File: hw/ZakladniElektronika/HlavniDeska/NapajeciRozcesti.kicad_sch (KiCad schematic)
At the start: 32 parts, among them Q1 Q_PMOS_DGS, Q2 Q_PMOS_DGS, U11 150k, U12 100k, U13 TPS61088RHLR, U14 100k, U15 2N7002, U16 LD39200, U17 33n, U18 150k, U19 22u, U20 4.7u, U21 10uf, U22 22u, U23 100k, U24 2N7002, U25 3.92k, U26 10n, U27 2.2u, U28 22u, U29 100p, U3 22u, U30 56k, U31 17.4k, U32 150k, U5 10uf, U6 100n, U7 1.2u, U8 4.7u, U9 100n

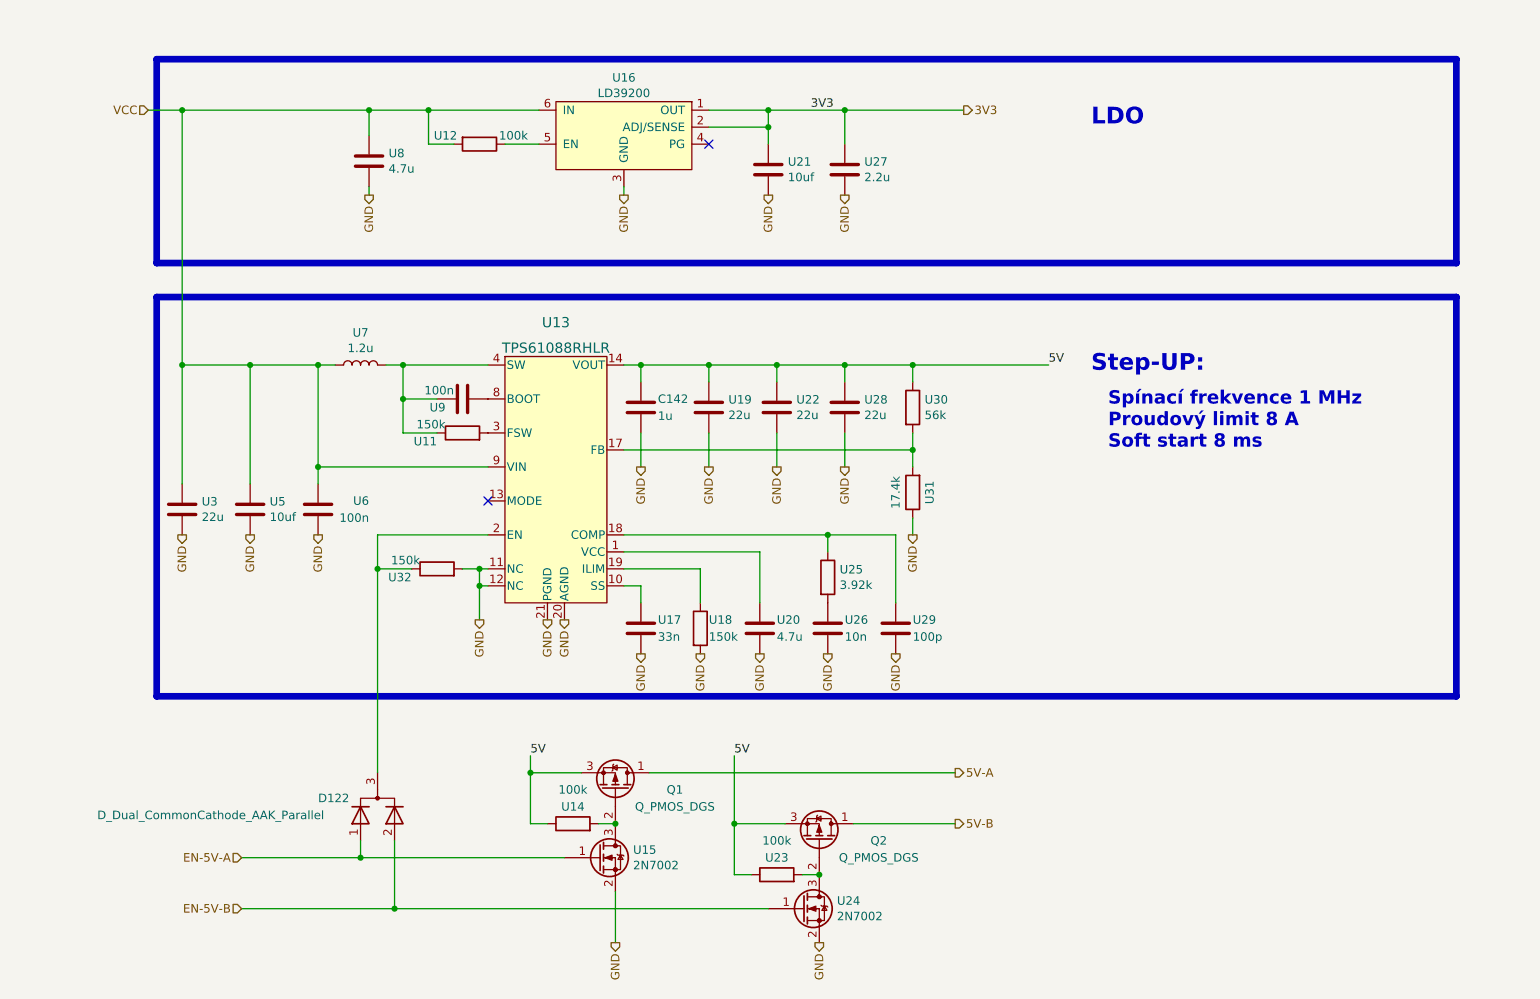
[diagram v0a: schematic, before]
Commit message: WIP
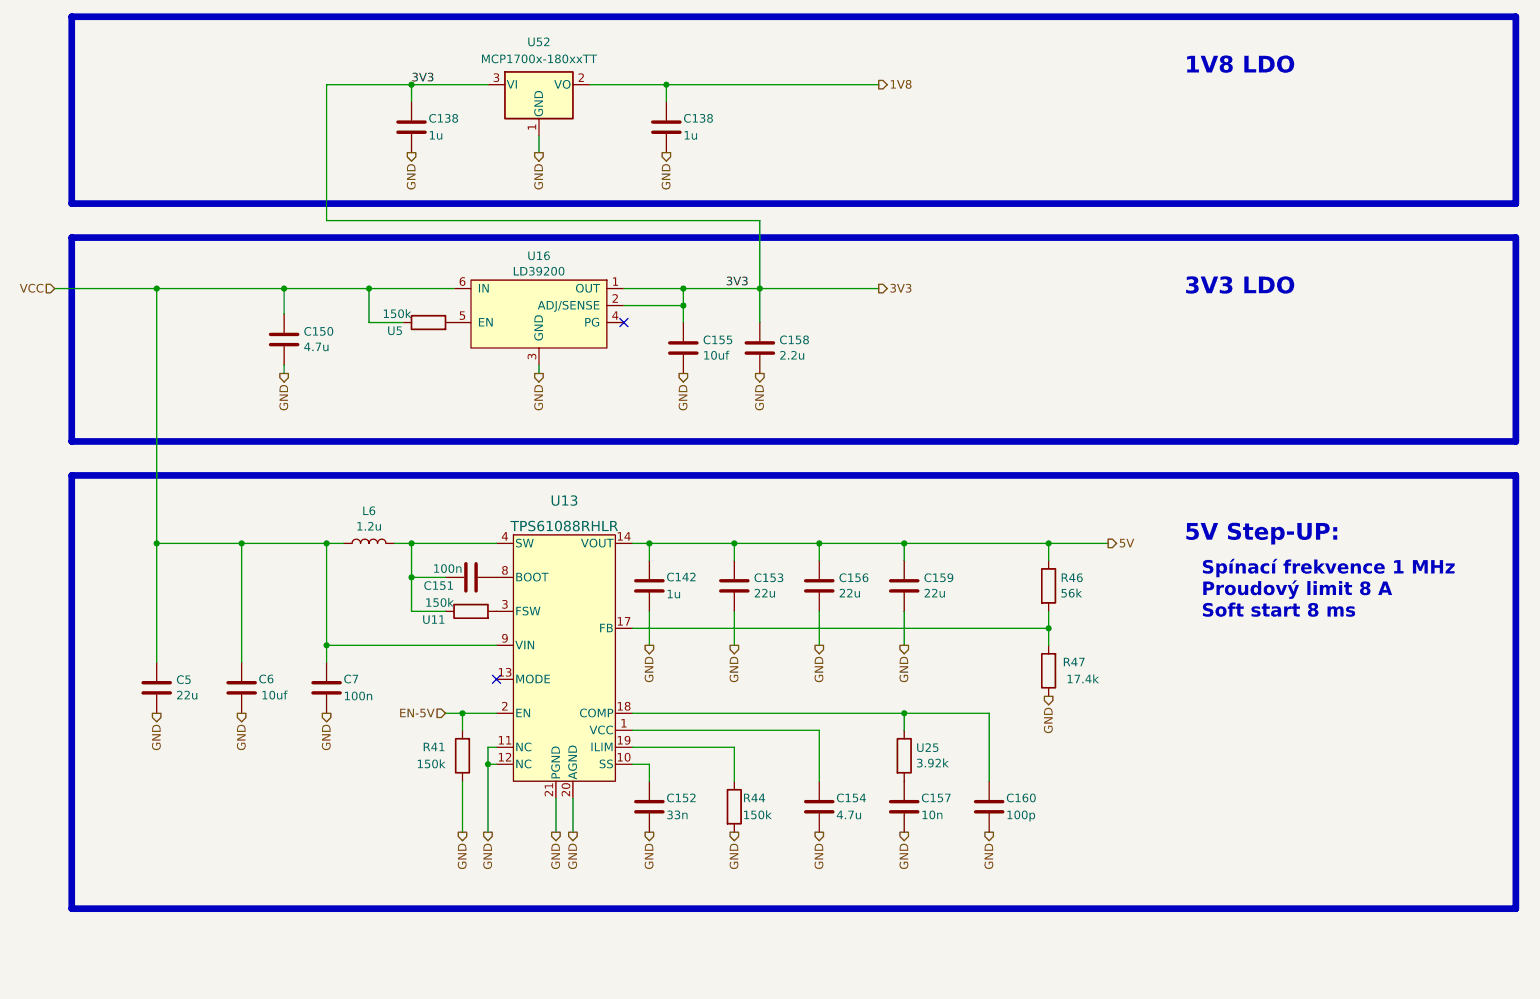
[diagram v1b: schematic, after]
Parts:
- removed D122: D_Dual_CommonCathode_AAK_Parallel, Package_TO_SOT_SMD:SOT-723, symbol Device:D_Dual_CommonCathode_AAK_Parallel
- removed Q1, Q2: Q_PMOS_DGS, RBCX:JMSL0302AU, symbol Device:Q_PMOS_DGS
- removed U12, U14, U23: 100k, Resistor_SMD:R_0402_1005Metric, symbol B.B-rescue:R-Device-B.B-rescue-B.B-rescue
- removed U15, U24: 2N7002, Package_TO_SOT_SMD:SOT-23, symbol B.B-rescue:2N7002-Transistor_FET-B.B-rescue-B.B-rescue
- added C138 (x2): 1u, Resistor_SMD:R_0402_1005Metric, symbol Device:C
- added U5: 150k, Resistor_SMD:R_0402_1005Metric, symbol B.B-rescue:R-Device-B.B-rescue-B.B-rescue
- added U52: MCP1700x-180xxTT, Package_TO_SOT_SMD:SOT-23, symbol Regulator_Linear:MCP1700x-180xxTT
- C142: Basic/Extended (none) -> E; LCSC C52923 -> C1518208; info (none) -> 50V, X7R
- C150: renamed from U8; symbol B.B-rescue:C-Device-B.B-rescue-B.B-rescue -> Device:C
- C151: renamed from U9; symbol B.B-rescue:C-Device-B.B-rescue-B.B-rescue -> Device:C; Basic/Extended (none) -> B; LCSC C1525 -> C307331; info (none) -> 50V, X7R
- C152: renamed from U17; symbol B.B-rescue:C-Device-B.B-rescue-B.B-rescue -> Device:C
- C153: renamed from U19; symbol B.B-rescue:C-Device-B.B-rescue-B.B-rescue -> Device:C
- C154: renamed from U20; symbol B.B-rescue:C-Device-B.B-rescue-B.B-rescue -> Device:C
- C155: renamed from U21; symbol B.B-rescue:C-Device-B.B-rescue-B.B-rescue -> Device:C
- C156: renamed from U22; symbol B.B-rescue:C-Device-B.B-rescue-B.B-rescue -> Device:C
- C157: renamed from U26; symbol B.B-rescue:C-Device-B.B-rescue-B.B-rescue -> Device:C
- C158: renamed from U27; symbol B.B-rescue:C-Device-B.B-rescue-B.B-rescue -> Device:C
- C159: renamed from U28; symbol B.B-rescue:C-Device-B.B-rescue-B.B-rescue -> Device:C
- C160: renamed from U29; symbol B.B-rescue:C-Device-B.B-rescue-B.B-rescue -> Device:C
- C5: renamed from U3; symbol B.B-rescue:C-Device-B.B-rescue-B.B-rescue -> Device:C
- C6: renamed from U5; symbol B.B-rescue:C-Device-B.B-rescue-B.B-rescue -> Device:C
- C7: renamed from U6; symbol B.B-rescue:C-Device-B.B-rescue-B.B-rescue -> Device:C; Basic/Extended (none) -> B; LCSC C1525 -> C307331; info (none) -> 50V, X7R
- renumbered U7 to L6, U32 to R41, U18 to R44, U30 to R46, U31 to R47
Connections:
- net 3V3: now also C138.1, U52.3 (VI)
- net GND: now also R41.1, C138.2, C138.2, U52.1 (GND); no longer R41.2
- net VCC: now also U5.1
- net EN-5V: now reaches U13.2 (EN)
- net EN-5V: now also R41.2; no longer R41.1
- net at U16.5 (EN): now also U5.2
- new net 1V8: C138.1, U52.2 (VO)
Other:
- note added: "1V8 LDO"
- note added: "3V3 LDO"
- note added: "5V Step-UP:"
- note removed: "LDO"
- note removed: "Step-UP:"
- moved on the sheet: C142, C150, C151, C152, C153, C154, C155, C156, C157, C158, C159, C160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
